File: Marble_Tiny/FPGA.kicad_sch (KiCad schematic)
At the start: 43 parts, among them T1 BSS138LT1G, T2 BSS138LT1G, U1 XC7A35T-CSG325, U28 24AA256UID-I_ST

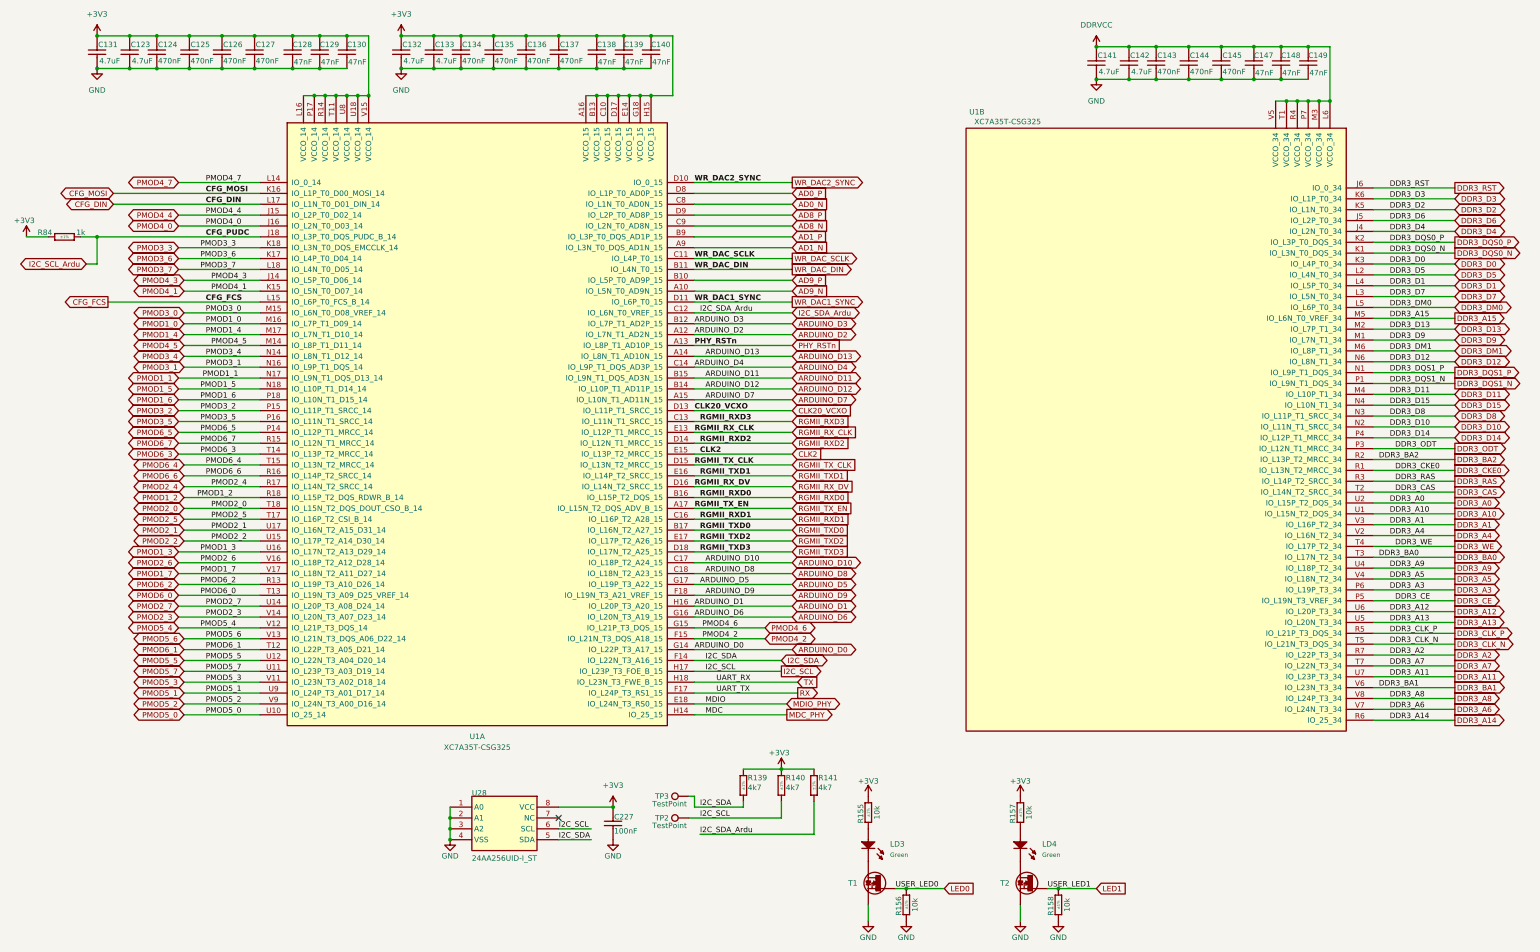
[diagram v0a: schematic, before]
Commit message: ready for the final review
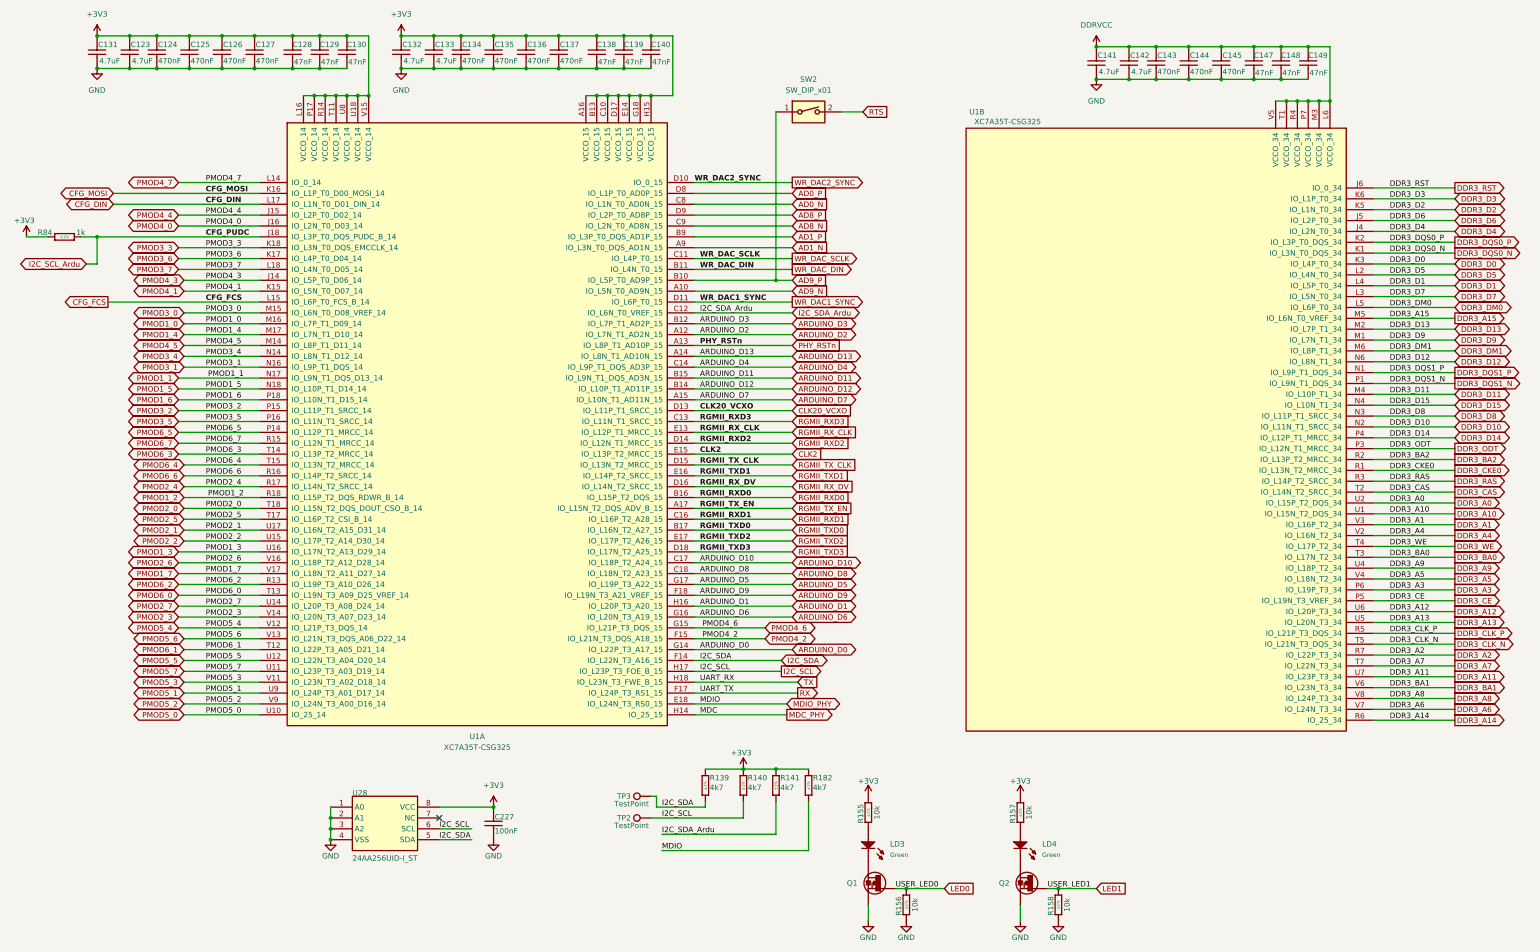
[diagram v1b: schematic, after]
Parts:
- added R182: R0402_4K7_1%_0.0625W_100PPM, Resistors SMD:RESC1005X40N, symbol Resistors SMD:R0402_4K7_1%_0.0625W_100PPM
- added SW2: SW_DIP_x01, Switches:SW_OMRON_A6SN-1101, symbol Switch:SW_DIP_x01
- renumbered T1 to Q1, T2 to Q2
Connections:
- net +3V3: now also R182.2
- net AD9_P: now also SW2.1
- net MDIO_PHY: now also R182.1
- new net RTS: SW2.2
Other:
- moved on the sheet: C227, R139, R140, R141, TP2, TP3, U28
